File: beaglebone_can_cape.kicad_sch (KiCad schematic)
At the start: 21 parts, among them J1 DCAN0, J2 DCAN1, J3 DTM15-12PA, P8 BeagleBone_Black_Header, P9 BeagleBone_Black_Header, U1 TCAN332, U2 TCAN332, U3 LMR51430

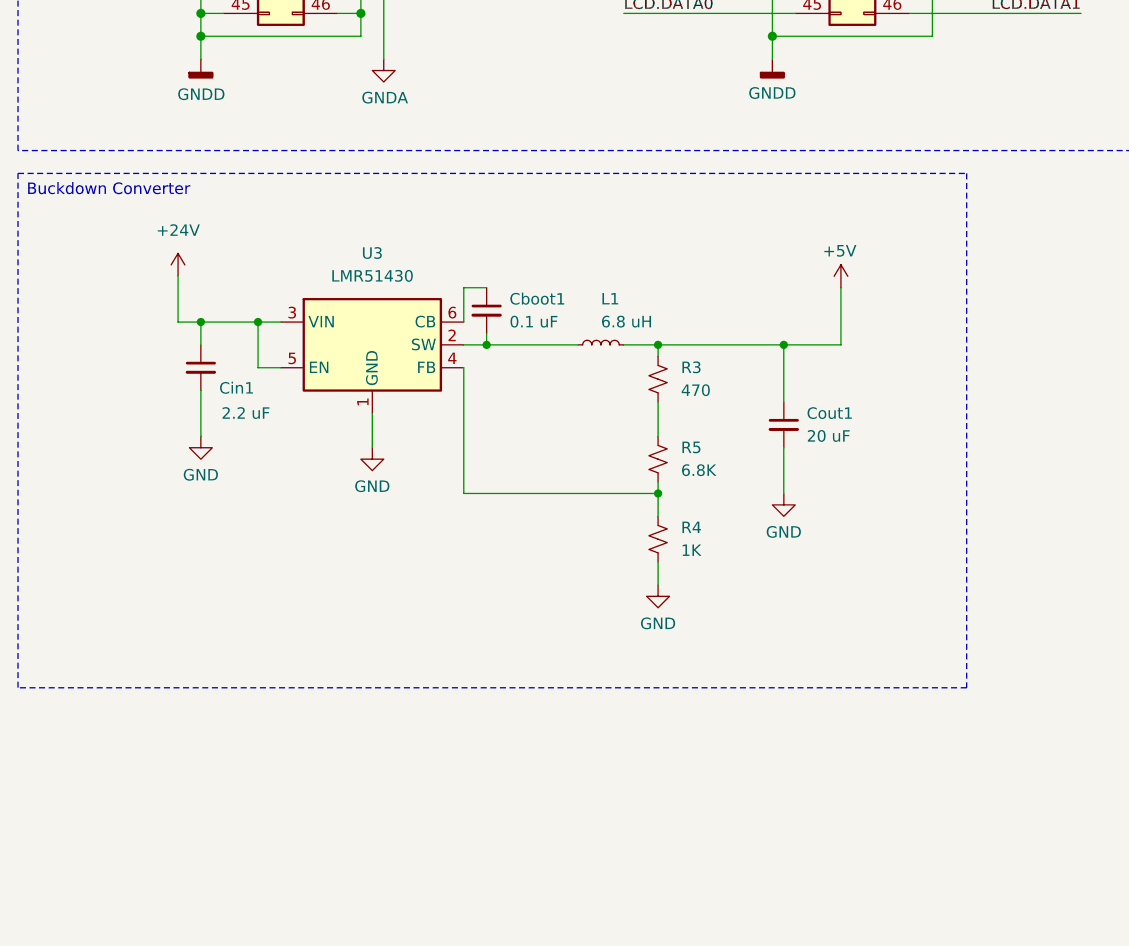
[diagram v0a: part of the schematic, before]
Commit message: taking break, letting Nash cook
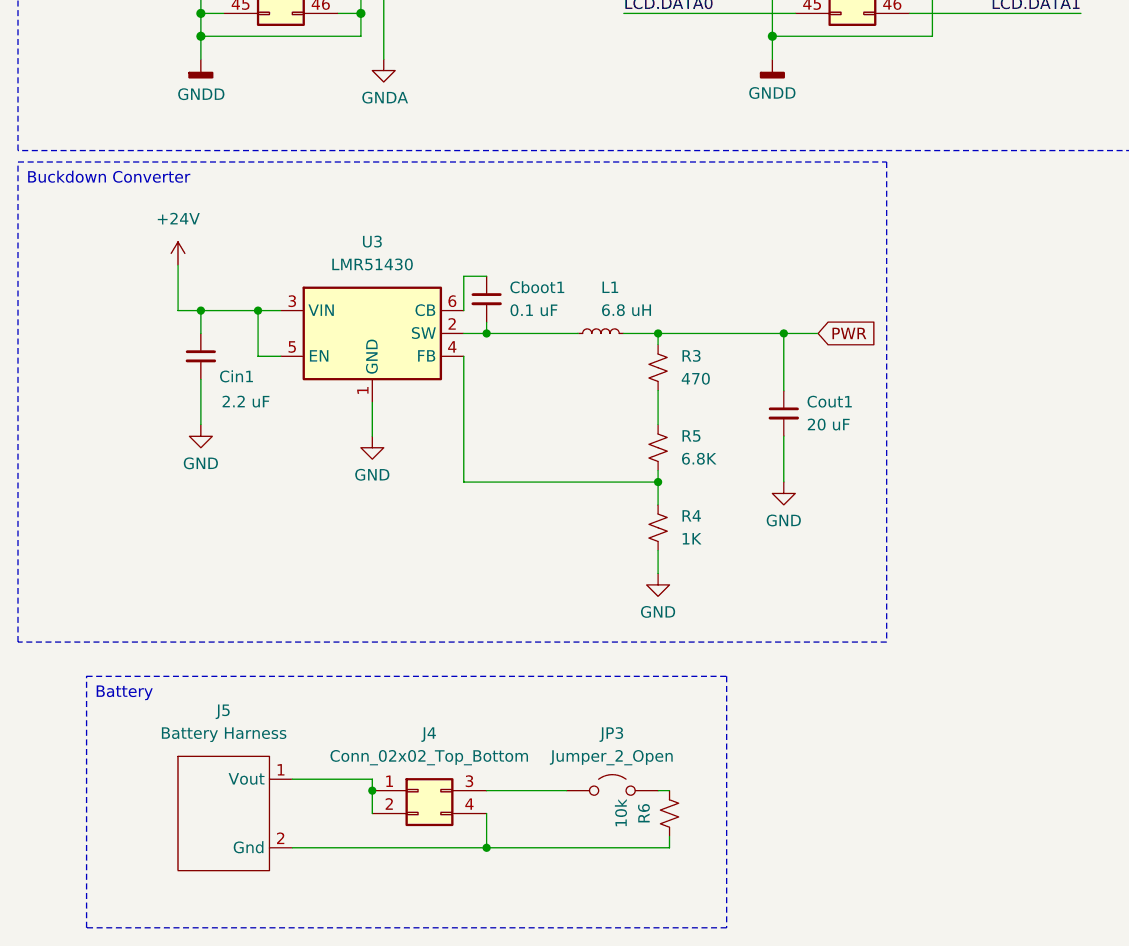
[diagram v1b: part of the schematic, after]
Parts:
- added J4: Conn_02x02_Top_Bottom, Connector_PinHeader_2.54mm:PinHeader_2x02_P2.54mm_Vertical, symbol Connector_Generic:Conn_02x02_Top_Bottom
- added J5: Battery Harness, SeniorDesign:BatteryHolder, symbol Senior_Design:BatteryHolder
- added JP3: Jumper_2_Open, symbol Jumper:Jumper_2_Open
- added R6: 10k, Resistor_SMD:R_0805_2012Metric, symbol Device:R_Small_US
- J3: footprint Senior Design:TE_DTM15-12PA -> DTM15-12PA:TE_DTM15-12PA
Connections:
- net +5V: no longer Cout1.1, L1.2, R3.1
- net PWR: now also Cout1.1, L1.2, R3.1
- new net: J4.1 (Pin_1), J4.2 (Pin_2), J5.1 (Vout)
- new net: J4.3 (Pin_3), JP3.1 (A)
- new net: J4.4 (Pin_4), J5.2 (Gnd), R6.2
- new net: JP3.2 (B), R6.1
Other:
- moved on the sheet: Cboot1, Cin1, Cout1, L1, R3, R4, R5, U3
